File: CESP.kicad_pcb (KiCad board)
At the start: 2 copper layers, 55.9 x 44.7 mm, 9 parts

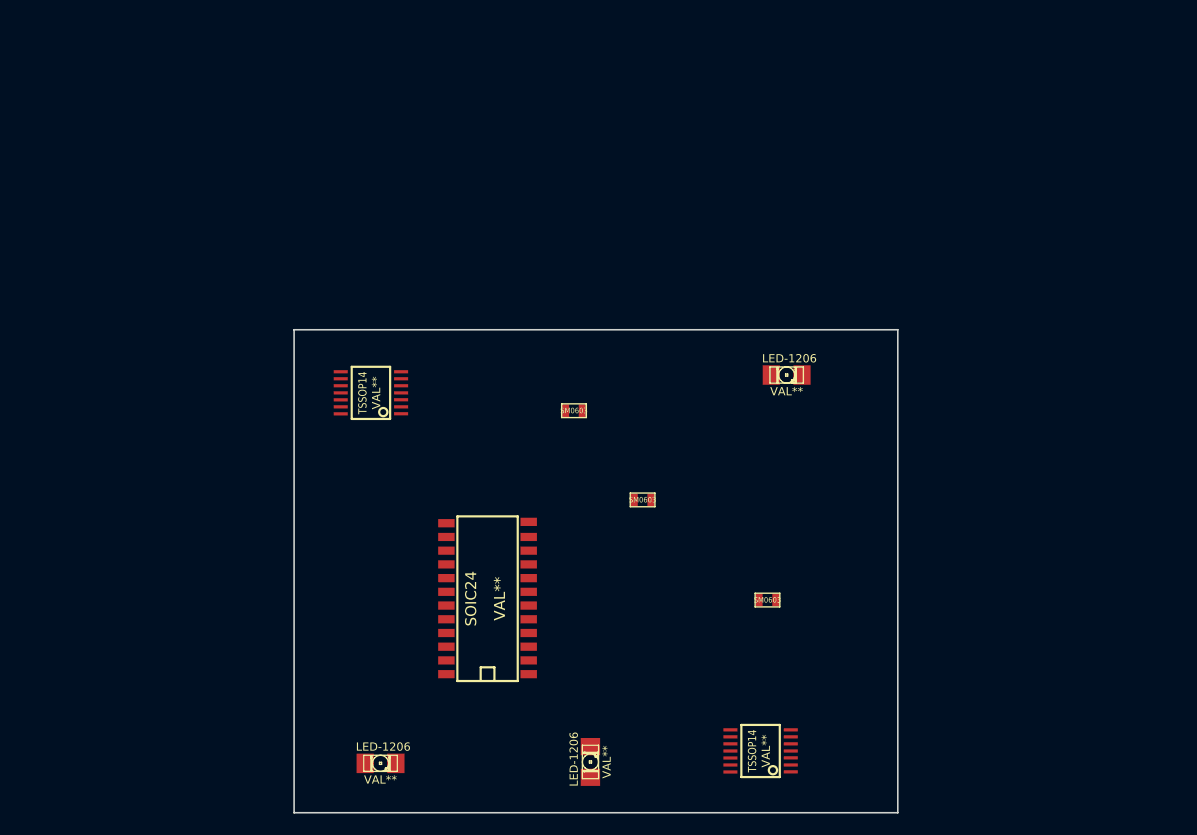
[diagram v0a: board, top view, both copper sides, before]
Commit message: Soldering practice board slapped together
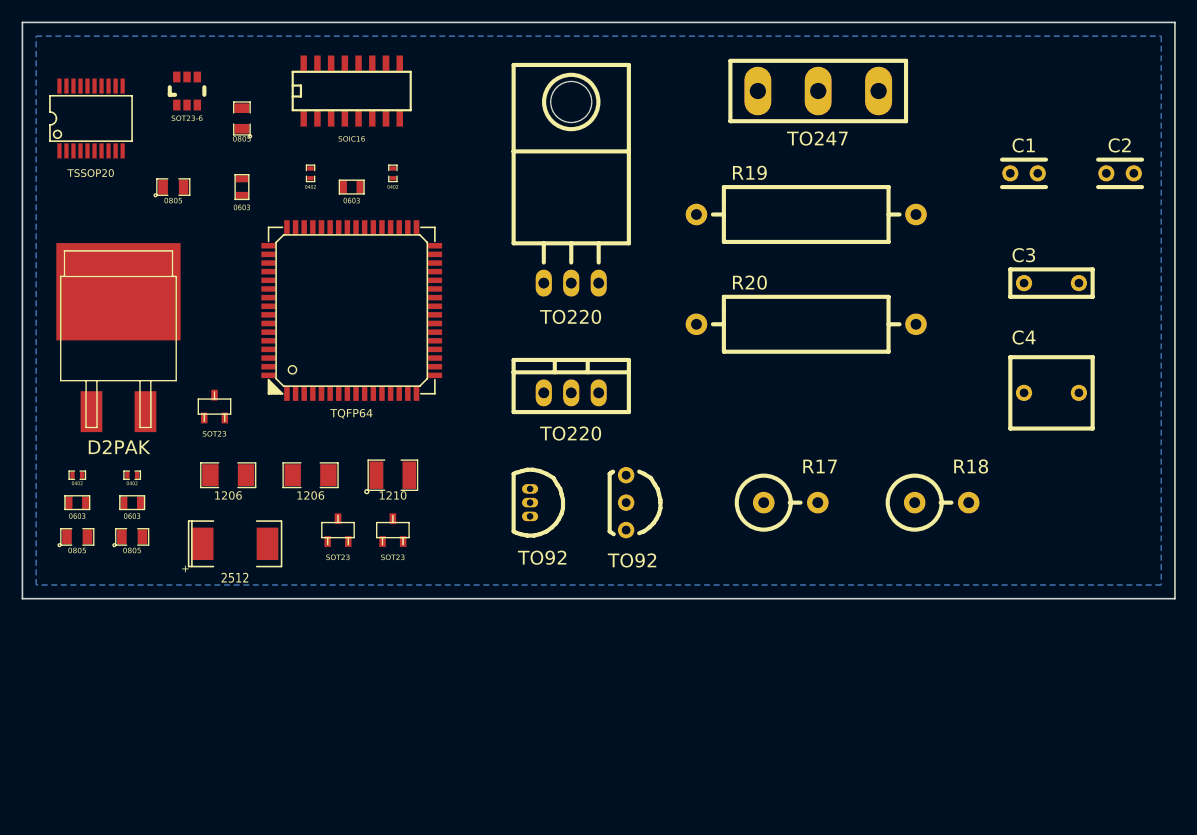
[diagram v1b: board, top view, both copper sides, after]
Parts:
- removed LED-1206 (x3): VAL**, LED-1206
- removed SM0603 (x3): Val**, SM0603
- removed SOIC24: VAL**, SOIC24
- removed TSSOP14 (x2): VAL**, TSSOP14
- added C1: C 2.5, Capacitors_ThroughHole:Capacitor4x3RM2.5, F.Cu at (222.2, 81.3)
- added C2: C 2.5, Capacitors_ThroughHole:Capacitor4x3RM2.5, F.Cu at (231.1, 81.3)
- added C3: C 5, Capacitors_ThroughHole:Capacitor7x2.5RM5, F.Cu at (223.5, 91.4)
- added C4: C 5, Capacitors_ThroughHole:Capacitor7.5x6.5RM5, F.Cu at (223.5, 101.6)
- added IC1: SOT23-6, Housings_SOT-23_SOT-143_TSOT-6:TSOT6-MK06A-Housing, F.Cu at (146.1, 73.7)
- added IC2: TSSOP20, SSOP_Packages:SSOP-20, F.Cu at (137.2, 76.2)
- added IC3: SOIC16, SOIC_Packages:SOIC-16_Narrow, F.Cu at (161.3, 73.7)
- added IC4: TQFP64, QFP:tqfp64-08, F.Cu at (161.3, 94.0)
- added Q1: SOT23, Transistors_SMD:sot23, F.Cu at (160.0, 114.3)
- added Q2: D2PAK, Transistors_SMD:sot404, F.Cu at (139.7, 97.8)
- added Q3: TO92, Housings_TO-92:TO-92-Free-inline-narrow-oval, F.Cu at (177.8, 111.8)
- added Q4: TO92, Housings_TO-92:TO-92-Free-inline-wide, F.Cu at (186.7, 111.8)
- added Q5: TO220, Transistors_TO-220:TO-220_Neutral123_Horizontal, F.Cu at (181.6, 91.4)
- added Q6: TO220, Transistors_TO-220:TO-220_Neutral123_Vertical, F.Cu at (181.6, 101.6)
- added Q7: TO247, Transistors_TO-247:TO-247_Vertical_Neutral123, F.Cu at (204.5, 73.7)
- added Q8: SOT23, Transistors_SMD:sot23, F.Cu at (165.1, 114.3)
- added Q9: SOT23, Transistors_SMD:sot23, F.Cu at (148.6, 102.9)
- added R1: 0402, SMD_Packages:SM0402, F.Cu at (135.9, 109.2)
- added R10: 0805, SMD_Packages:SM0805, F.Cu at (141.0, 114.9)
- added R11: 0805, SMD_Packages:SM0805, F.Cu at (144.8, 82.5)
- added R12: 0805, SMD_Packages:SM0805, F.Cu at (151.1, 76.2)
- added R13: 1206, SMD_Packages:SM1206, F.Cu at (149.9, 109.2)
- added R14: 1206, SMD_Packages:SM1206, F.Cu at (157.5, 109.2)
- added R15: 1210, SMD_Packages:SM1210, F.Cu at (165.1, 109.2)
- added R16: 2512, SMD_Packages:SM2512, F.Cu at (150.5, 115.6)
- added R17: R VERT, Resistors_ThroughHole:Resistor_Vertical_RM5mm, F.Cu at (201.9, 111.8)
- added R18: R VERT, Resistors_ThroughHole:Resistor_Vertical_RM5mm, F.Cu at (215.9, 111.8)
- added R19: R HOR, Resistors_ThroughHole:Resistor_Horizontal_RM20mm, F.Cu at (203.2, 85.1)
- added R2: 0402, SMD_Packages:SM0402, F.Cu at (141.0, 109.2)
- added R20: R HORI, Resistors_ThroughHole:Resistor_Horizontal_RM20mm, F.Cu at (203.2, 95.2)
- added R3: 0402, SMD_Packages:SM0402, F.Cu at (157.5, 81.3)
- added R4: 0402, SMD_Packages:SM0402, F.Cu at (165.1, 81.3)
- added R5: 0603, SMD_Packages:SM0603, F.Cu at (135.9, 111.8)
- added R6: 0603, SMD_Packages:SM0603, F.Cu at (141.0, 111.8)
- added R7: 0603, SMD_Packages:SM0603, F.Cu at (151.1, 82.5)
- added R8: 0603, SMD_Packages:SM0603, F.Cu at (161.3, 82.5)
- added R9: 0805, SMD_Packages:SM0805, F.Cu at (135.9, 114.9)
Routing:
- added copper zone on B.Cu, net GND
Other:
- board size 55.9 x 44.7 mm -> 106.7 x 53.3 mm
- board text removed: "NOTE: THIS IS JUST A TEST BOARD REMOVE ALL COMPONENTS AND CREATE YOUR OWN INCLUDE SCHEMATIC HOOKUPS/NETLIST"
